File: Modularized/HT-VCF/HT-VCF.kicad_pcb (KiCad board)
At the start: 2 copper layers, 63.5 x 50.8 mm, 29 parts

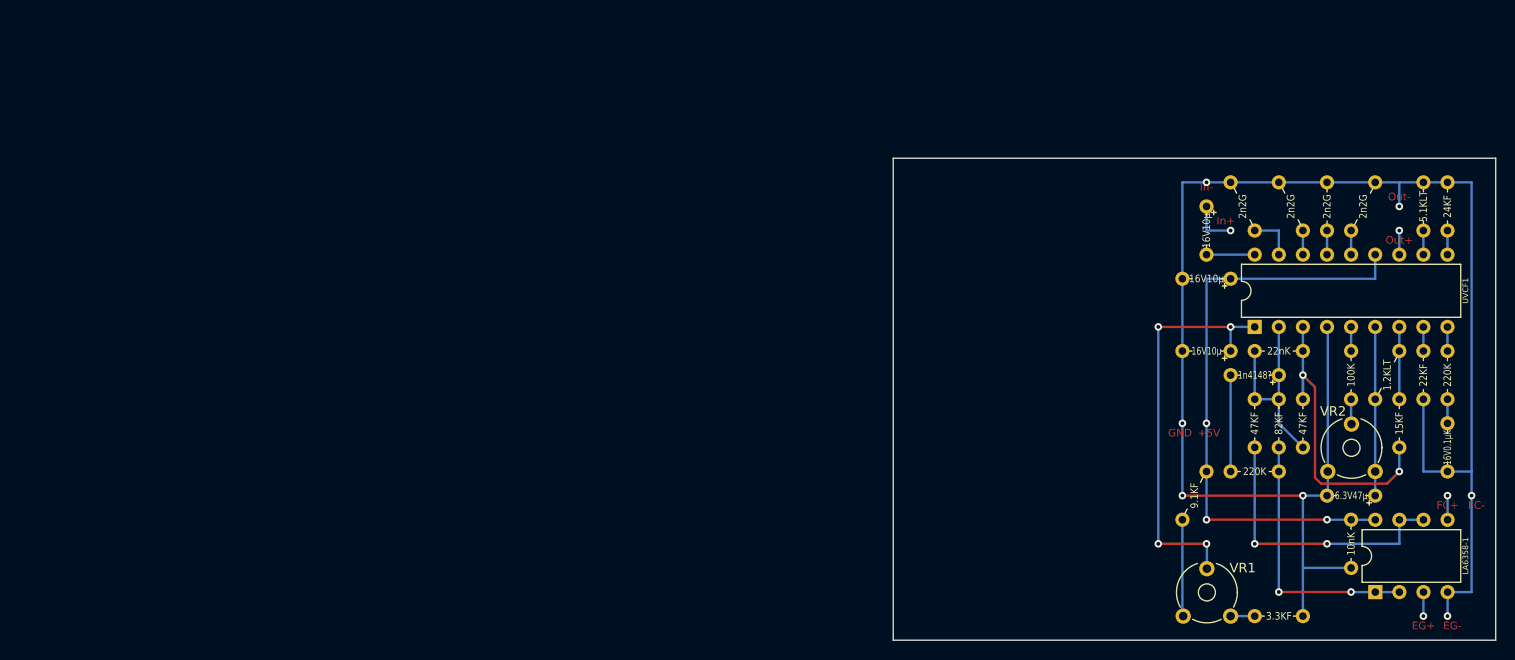
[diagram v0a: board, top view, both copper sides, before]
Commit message: save point
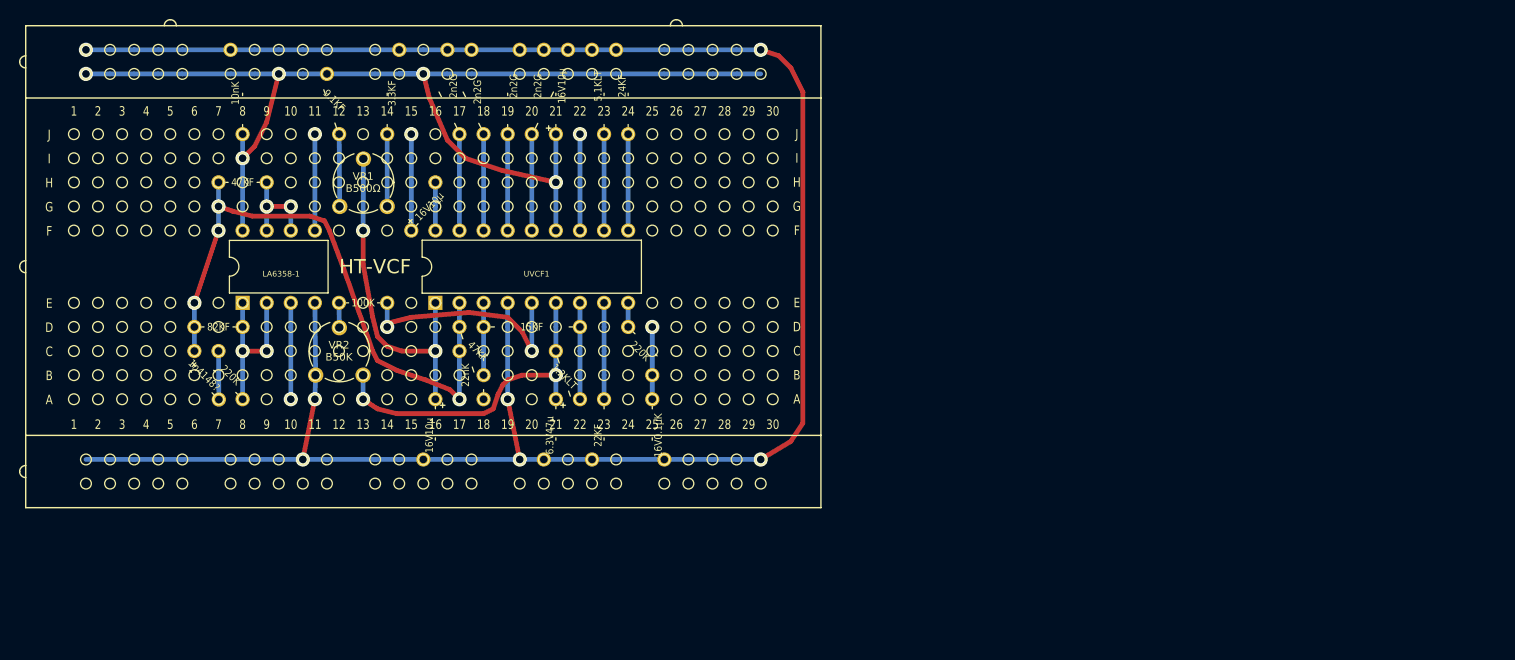
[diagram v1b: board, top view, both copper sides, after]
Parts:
- added +5VA: REF**, MyKi_TH_Board_Features:Labled-Circle, F.Cu at (85.1, 49.5)
- added AG: REF**, MyKi_TH_Board_Features:Labled-Circle, F.Cu at (85.1, 47.0)
- added Cut: REF**, MyKi_TH_Board_Features:Labled-Circle, F.Cu at (106.7, 58.4)
- added Env: REF**, MyKi_TH_Board_Features:Labled-Circle, F.Cu at (104.1, 86.4)
- added In: REF**, MyKi_TH_Board_Features:Labled-Circle, F.Cu at (116.8, 58.4)
- added OUT: REF**, MyKi_TH_Board_Features:Labled-Circle, F.Cu at (137.2, 55.9)
- added Reso: REF**, MyKi_TH_Board_Features:Labled-Circle, F.Cu at (144.8, 76.2)
- added VAL**: REF**, MyKi_TH_Board_Features:breadboard-30-4Rail, F.Cu at (121.9, 69.8)
- LA6358-1: value NJM4558 -> LA6358
- R13: footprint MyKi_Generics:200Mil_2TH_Generic -> MyKi_Generics:400Mil_2TH_Generic
- R5: footprint MyKi_Generics:200Mil_2TH_Generic -> MyKi_Generics:200Mil_2TH_Dn1_Generic
- VR1, VR2: footprint Potentiometers:Potentiometer_Trimmer_Piher_PT-6v_Horizontal -> MyKi_Generics:200x200Mil_3TH_TrimPot
- moved C11 127.4 mm to (101.6, 50.8), turned to 270 degrees
- moved LA6358-1 123.2 mm to (101.6, 73.7)
- moved D1 115.3 mm to (95.5, 80.3), turned to 315 degrees
- moved R11 110.0 mm to (101.6, 76.2), turned to 180 degrees
- moved R10 109.5 mm to (101.6, 83.8), turned to 135 degrees
- moved R12 107.8 mm to (104.1, 61.0), turned to 180 degrees
- moved VR2 107.2 mm to (114.3, 81.3)
- moved R4 104.6 mm to (116.8, 55.9), turned to 90 degrees
- moved R3 101.8 mm to (110.0, 50.5), turned to 315 degrees
- moved R7 101.7 mm to (116.8, 73.7), turned to 180 degrees
- moved VR1 98.8 mm to (116.8, 63.5)
- moved R5 89.8 mm to (124.5, 76.2), turned to 315 degrees
- moved C4 87.0 mm to (127.0, 55.9)
- moved C5 87.0 mm to (129.5, 55.9)
- moved R1 87.0 mm to (139.7, 50.8)
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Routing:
- net +5VA: track 63.5 -> 123.9 mm, vias 3 -> 5
- net GNDA: track 178.0 -> 223.1 mm
- net Net-(C8-Pad2): track 21.4 -> 65.2 mm, vias 0 -> 4
- net Net-(C8-Pad1): track 33.7 -> 7.62 mm, vias 2 -> 0
- net Net-(R7-Pad1): track 2.54 -> 25.1 mm, vias 0 -> 2
- net Net-(LA6358-1-Pad6): track 30.5 -> 10.2 mm
- net Net-(C10-Pad1): track 17.8 -> 35.5 mm, vias 0 -> 2
- net Net-(LA6358-1-Pad1): track 28.0 -> 17.8 mm
- net /VBB: track 43.3 -> 35.6 mm, vias 4 -> 2
- net /ENV: track 2.53 -> 10.2 mm
- net Net-(R2-Pad2): track 2.54 -> 10.2 mm
- net Net-(R1-Pad2): track 2.54 -> 10.2 mm
- net Net-(C6-Pad1): track 2.54 -> 10.2 mm
- net Net-(C5-Pad1): track 2.54 -> 10.2 mm
- net Net-(C4-Pad1): track 2.54 -> 10.2 mm
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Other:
- board outline removed
- net class Default: trace_width 0.25 -> 0.5; via_dia 0.8 -> 1.5; via_drill 0.4 -> 0.8
- rule pad_to_mask_clearance: 0.2 -> 0
- rule trace_min: 0.2 -> 0.5
- rule via_min_drill: 0.3 -> 0.8
- rule via_min_size: 0.4 -> 1.5
- board text added: "HT-VCF"
- board text removed: "+5V"
- board text removed: "EG+"
- board text removed: "EG-"
- board text removed: "FC+"
- board text removed: "FC-"
- board text removed: "GND"
- board text removed: "In+"
- board text removed: "In-"
- board text removed: "Out+"
- board text removed: "Out-"
